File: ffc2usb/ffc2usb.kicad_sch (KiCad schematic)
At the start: 2 parts, among them J1 USB3_A, U1 62674-201121ALF

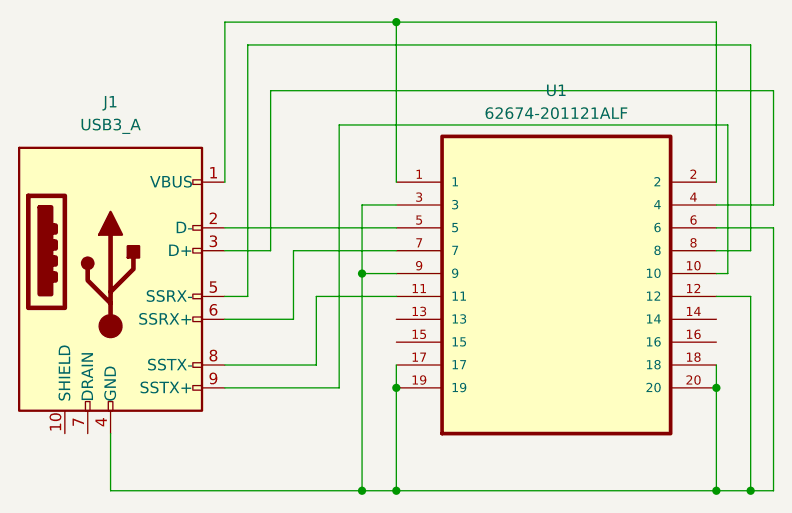
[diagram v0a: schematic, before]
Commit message: lceda project
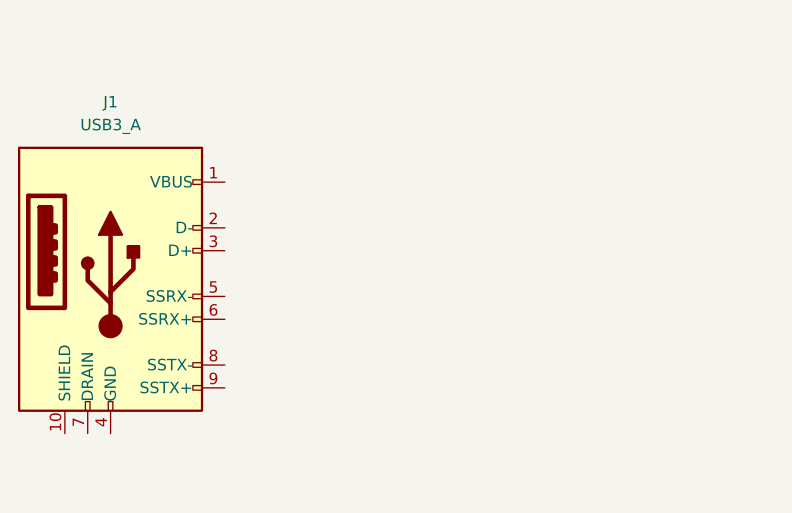
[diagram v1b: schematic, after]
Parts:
- removed U1: 62674-201121ALF, 62674-201121ALF:FCI_62674-201121ALF, symbol 20pin_ffc_connnector:62674-201121ALF
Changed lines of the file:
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@@
 (kicad_sch (version 20230121) (generator eeschema)
   (paper "A4")
-  (junction (at 153.67 106.68) (diameter 0) (color 0 0 0 0)
-  )
-  (junction (at 157.48 118.11) (diameter 0) (color 0 0 0 0)
-  )
-  (junction (at 118.11 106.68) (diameter 0) (color 0 0 0 0)
-  )
-  (junction (at 153.67 118.11) (diameter 0) (color 0 0 0 0)
-  )
-  (junction (at 118.11 118.11) (diameter 0) (color 0 0 0 0)
-  )
-  (junction (at 118.11 66.04) (diameter 0) (color 0 0 0 0)
-  )
-  (junction (at 114.3 93.98) (diameter 0) (color 0 0 0 0)
-  )
-  (junction (at 114.3 118.11) (diameter 0) (color 0 0 0 0)
-  )
-  (wire (pts (xy 104.14 91.44) (xy 99.06 91.44))
-    (stroke (width 0) (type default))
-  )
-  (wire (pts (xy 118.11 91.44) (xy 106.68 91.44))
-    (stroke (width 0) (type default))
-  )
-  (wire (pts (xy 153.67 93.98) (xy 154.94 93.98))
-    (stroke (width 0) (type default))
-  )
-  (wire (pts (xy 157.48 118.11) (xy 153.67 118.11))
-    (stroke (width 0) (type default))
-  )
-  (wire (pts (xy 99.06 66.04) (xy 99.06 83.82))
-    (stroke (width 0) (type default))
-  )
-  (wire (pts (xy 118.11 104.14) (xy 118.11 106.68))
-    (stroke (width 0) (type default))
-  )
-  (wire (pts (xy 118.11 118.11) (xy 114.3 118.11))
-    (stroke (width 0) (type default))
-  )
-  (wire (pts (xy 153.67 104.14) (xy 153.67 106.68))
-    (stroke (width 0) (type default))
-  )
-  (wire (pts (xy 114.3 93.98) (xy 114.3 118.11))
-    (stroke (width 0) (type default))
-  )
-  (wire (pts (xy 99.06 88.9) (xy 118.11 88.9))
-    (stroke (width 0) (type default))
-  )
-  (wire (pts (xy 157.48 91.44) (xy 157.48 68.58))
-    (stroke (width 0) (type default))
-  )
-  (wire (pts (xy 153.67 88.9) (xy 160.02 88.9))
-    (stroke (width 0) (type default))
-  )
-  (wire (pts (xy 111.76 106.68) (xy 99.06 106.68))
-    (stroke (width 0) (type default))
-  )
-  (wire (pts (xy 109.22 96.52) (xy 109.22 104.14))
-    (stroke (width 0) (type default))
-  )
-  (wire (pts (xy 157.48 68.58) (xy 101.6 68.58))
-    (stroke (width 0) (type default))
-  )
-  (wire (pts (xy 114.3 86.36) (xy 114.3 93.98))
-    (stroke (width 0) (type default))
-  )
-  (wire (pts (xy 153.67 86.36) (xy 160.02 86.36))
-    (stroke (width 0) (type default))
-  )
-  (wire (pts (xy 111.76 77.47) (xy 111.76 106.68))
-    (stroke (width 0) (type default))
-  )
-  (wire (pts (xy 153.67 96.52) (xy 157.48 96.52))
-    (stroke (width 0) (type default))
-  )
-  (wire (pts (xy 153.67 106.68) (xy 153.67 118.11))
-    (stroke (width 0) (type default))
-  )
-  (wire (pts (xy 118.11 106.68) (xy 118.11 118.11))
-    (stroke (width 0) (type default))
-  )
-  (wire (pts (xy 160.02 86.36) (xy 160.02 73.66))
-    (stroke (width 0) (type default))
-  )
-  (wire (pts (xy 118.11 96.52) (xy 109.22 96.52))
-    (stroke (width 0) (type default))
-  )
-  (wire (pts (xy 114.3 118.11) (xy 86.36 118.11))
-    (stroke (width 0) (type default))
-  )
-  (wire (pts (xy 99.06 96.52) (xy 101.6 96.52))
-    (stroke (width 0) (type default))
-  )
-  (wire (pts (xy 99.06 99.06) (xy 106.68 99.06))
-    (stroke (width 0) (type default))
-  )
-  (wire (pts (xy 154.94 77.47) (xy 111.76 77.47))
-    (stroke (width 0) (type default))
-  )
-  (wire (pts (xy 118.11 86.36) (xy 114.3 86.36))
-    (stroke (width 0) (type default))
-  )
-  (wire (pts (xy 153.67 83.82) (xy 153.67 66.04))
-    (stroke (width 0) (type default))
-  )
-  (wire (pts (xy 114.3 93.98) (xy 118.11 93.98))
-    (stroke (width 0) (type default))
-  )
-  (wire (pts (xy 153.67 91.44) (xy 157.48 91.44))
-    (stroke (width 0) (type default))
-  )
-  (wire (pts (xy 101.6 68.58) (xy 101.6 96.52))
-    (stroke (width 0) (type default))
-  )
-  (wire (pts (xy 118.11 66.04) (xy 118.11 83.82))
-    (stroke (width 0) (type default))
-  )
-  (wire (pts (xy 118.11 66.04) (xy 99.06 66.04))
-    (stroke (width 0) (type default))
-  )
-  (wire (pts (xy 154.94 93.98) (xy 154.94 77.47))
-    (stroke (width 0) (type default))
-  )
-  (wire (pts (xy 160.02 73.66) (xy 104.14 73.66))
-    (stroke (width 0) (type default))
-  )
-  (wire (pts (xy 160.02 118.11) (xy 157.48 118.11))
-    (stroke (width 0) (type default))
-  )
-  (wire (pts (xy 153.67 66.04) (xy 118.11 66.04))
-    (stroke (width 0) (type default))
-  )
-  (wire (pts (xy 109.22 104.14) (xy 99.06 104.14))
-    (stroke (width 0) (type default))
-  )
-  (wire (pts (xy 160.02 88.9) (xy 160.02 118.11))
-    (stroke (width 0) (type default))
-  )
-  (wire (pts (xy 106.68 91.44) (xy 106.68 99.06))
-    (stroke (width 0) (type default))
-  )
-  (wire (pts (xy 86.36 111.76) (xy 86.36 118.11))
-    (stroke (width 0) (type default))
-  )
-  (wire (pts (xy 153.67 118.11) (xy 118.11 118.11))
-    (stroke (width 0) (type default))
-  )
-  (wire (pts (xy 104.14 73.66) (xy 104.14 91.44))
-    (stroke (width 0) (type default))
-  )
-  (wire (pts (xy 157.48 96.52) (xy 157.48 118.11))
-    (stroke (width 0) (type default))
-  )
-  (symbol (lib_id "20pin_ffc_connnector:62674-201121ALF") (at 135.89 91.44 0) (unit 1)
-    (in_bom yes) (on_board yes) (dnp no) (fields_autoplaced)
-    (property "Reference" "U1" (at 135.89 73.66 0)
-      (effects (font (size 1.27 1.27)))
-    )
-    (property "Value" "62674-201121ALF" (at 135.89 76.2 0)
-      (effects (font (size 1.27 1.27)))
-    )
-    (property "Footprint" "62674-201121ALF:FCI_62674-201121ALF" (at 135.89 91.44 0)
-      (effects (font (size 1.27 1.27)) (justify bottom) hide)
-    )
-    (property "Datasheet" "" (at 135.89 91.44 0)
-      (effects (font (size 1.27 1.27)) hide)
-    )
-    (property "MPN" "62674-201121ALF" (at 135.89 91.44 0)
-      (effects (font (size 1.27 1.27)) (justify bottom) hide)
-    )
-    (property "OC_FARNELL" "1830629" (at 135.89 91.44 0)
-      (effects (font (size 1.27 1.27)) (justify bottom) hide)
-    )
-    (property "OC_NEWARK" "03M2161" (at 135.89 91.44 0)
-      (effects (font (size 1.27 1.27)) (justify bottom) hide)
-    )
-    (property "SUPPLIER" "FCI" (at 135.89 91.44 0)
-      (effects (font (size 1.27 1.27)) (justify bottom) hide)
-    )
-    (property "PACKAGE" "CONN-20POS" (at 135.89 91.44 0)
-      (effects (font (size 1.27 1.27)) (justify bottom) hide)
-    )
-    (pin "9")
-    (pin "20")
-    (pin "19")
-    (pin "1")
-    (pin "10")
-    (pin "13")
-    (pin "3")
-    (pin "2")
-    (pin "4")
-    (pin "17")
-    (pin "15")
-    (pin "5")
-    (pin "12")
-    (pin "11")
-    (pin "18")
-    (pin "14")
-    (pin "6")
-    (pin "8")
-    (pin "7")
-    (pin "16")
-    (instances
-      (project "ffc2usb"
-        (path "/9c1484d3-190d-4da9-a265-940fb3e31734"
-          (reference "U1") (unit 1)
-        )
-      )
-    )
-  )
   (symbol (lib_id "Connector:USB3_A") (at 86.36 93.98 0) (unit 1)
     (in_bom yes) (on_board yes) (dnp no) (fields_autoplaced)
